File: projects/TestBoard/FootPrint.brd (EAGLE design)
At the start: 100 x 80 mm, 14 parts

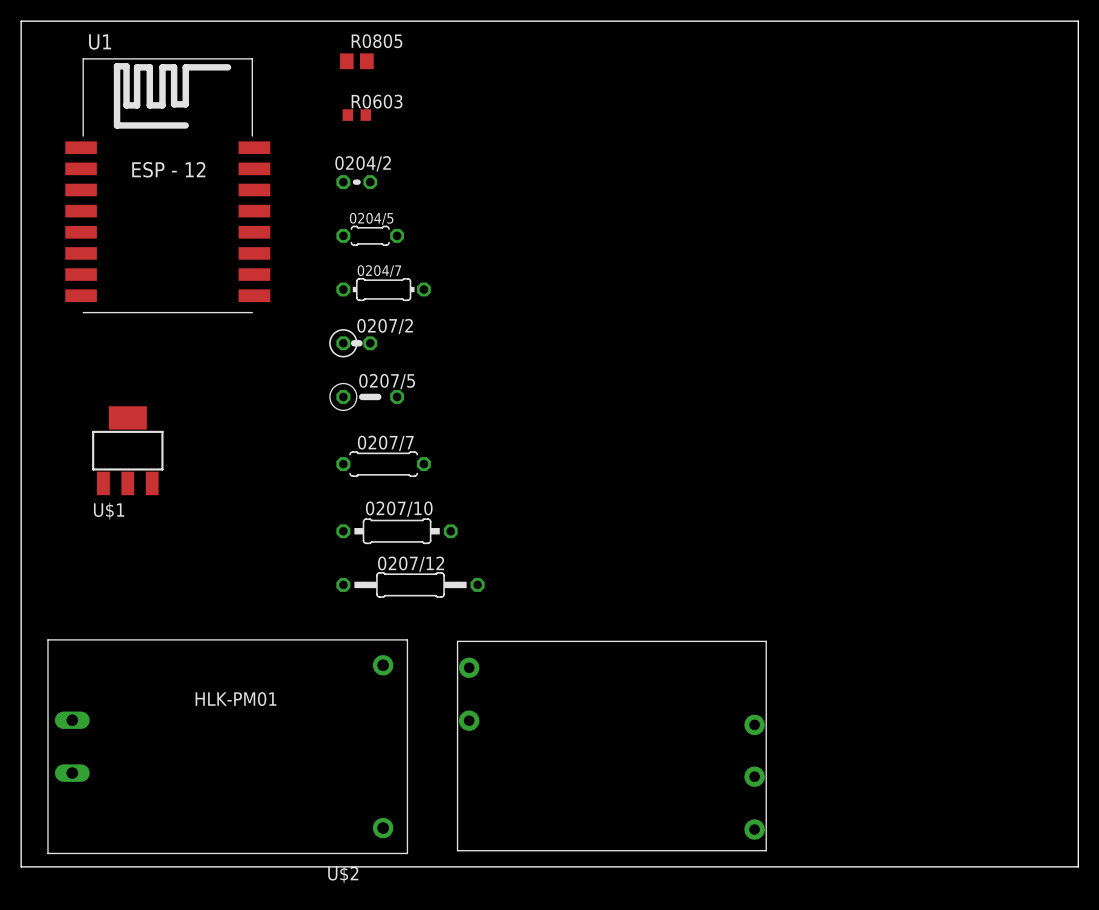
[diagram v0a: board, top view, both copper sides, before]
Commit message: 14-8-59
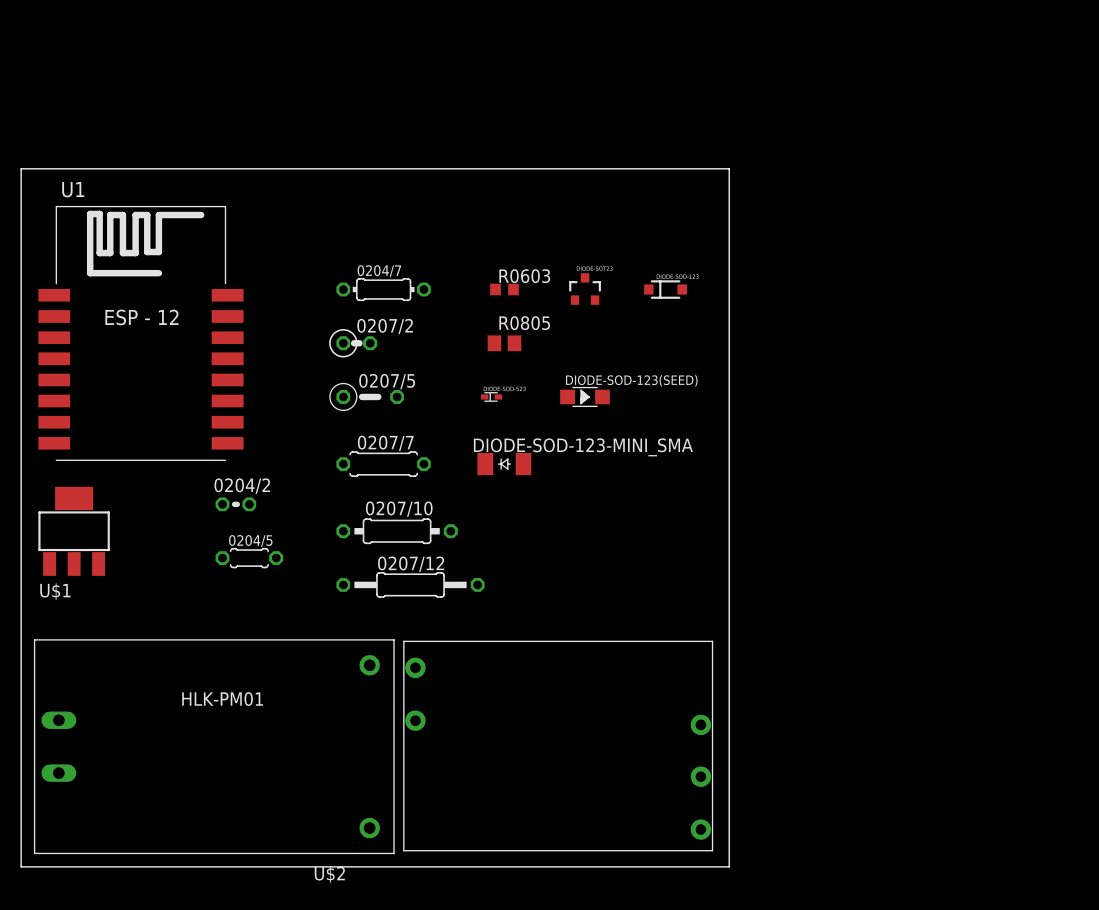
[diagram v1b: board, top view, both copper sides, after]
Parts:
- added DIODE-SOD-123: (no value), SparkFun-DiscreteSemi:SOD-123
- added DIODE-SOD-123(SEED): MMSD4148-sod123, Seeed-OPL-Diode:SOD-123
- added DIODE-SOD-123-MINI_SMA: CGRM4001-G, diode:SOD-123_MINI-SMA
- added DIODE-SOD-523: (no value), SparkFun-DiscreteSemi:SOD523
- added DIODE-SOT23: (no value), SparkFun-DiscreteSemi:SOT23-3
- moved 0204/5 32.6 mm to (21.6, 29.2)
- moved 0204/2 32.6 mm to (20.3, 34.3)
- moved R0805 30.1 mm to (45.7, 49.5)
- moved R0603 21.6 mm to (45.7, 54.6)
- moved U1 14.2 mm to (11.4, 48.3)
- moved U$1 9.16 mm to (5.08, 31.8)
- moved U$3 5.08 mm to (50.8, 11.4)
- moved U$2 1.27 mm to (17.8, 11.4)
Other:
- board size 100 x 80 mm -> 67 x 66 mm
